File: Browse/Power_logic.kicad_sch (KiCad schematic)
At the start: 12 parts

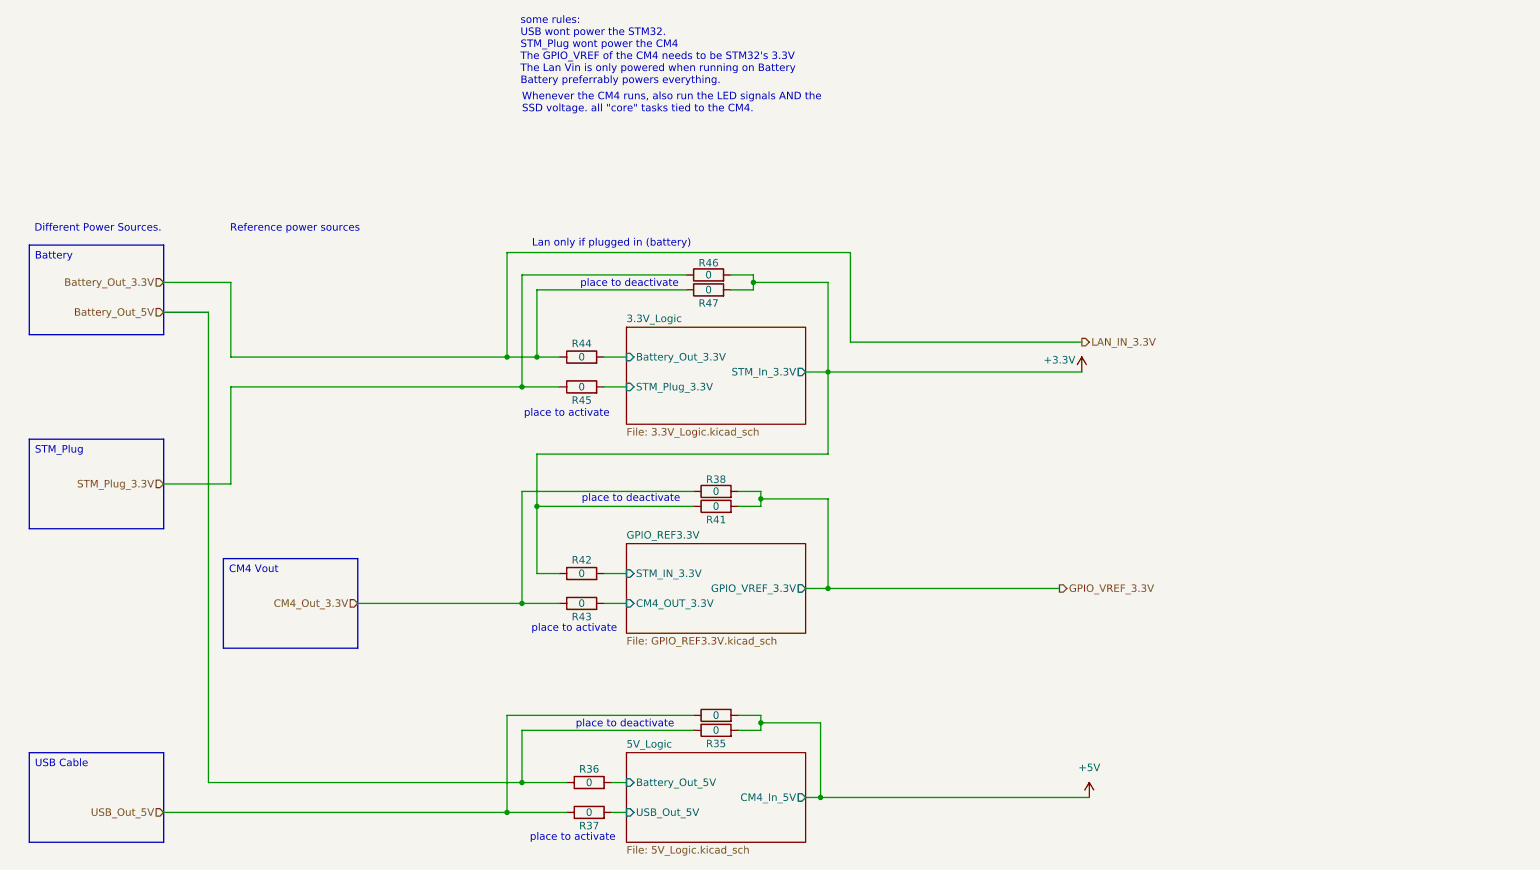
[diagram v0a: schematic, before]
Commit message: Deploying to gh-pages from @ Nautilus-UUV/nautilus-mainboard-PCB@5b07cf6af03655ef9ddad269b1edd5eb03bfa75f 🚀
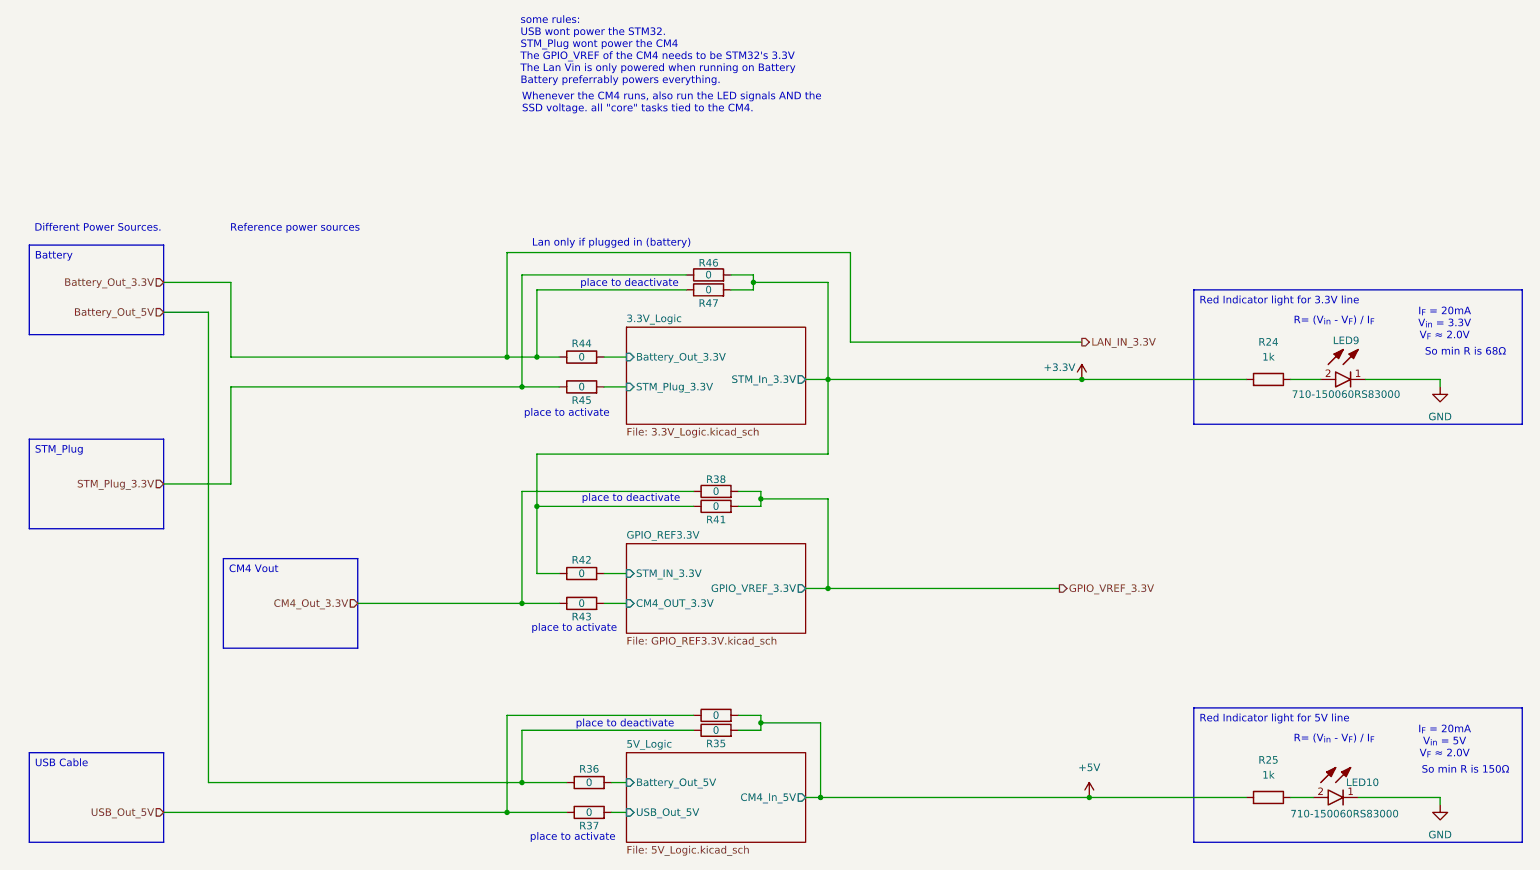
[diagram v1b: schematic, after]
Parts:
- added LED10, LED9: 710-150060RS83000, dz_dio:Wuerth_LED_150060RS83000, symbol #dzdb:s_dio/D-WURT-710-150060RS83000
- added R24, R25: 1k, Resistor_SMD:R_0603_1608Metric, symbol #dzdb:g_res/R-1k-0603
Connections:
- net +3.3V: now also R24.2
- net +5V: now also R25.2
- new net: LED10.2 (A), R25.1
- new net: LED9.2 (A), R24.1
- new net GND: LED10.1 (K), LED9.1 (K)
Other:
- note added: "I_{F} = 20mA V_{in} = 3.3V V_{F} ≈ 2.0V"
- note added: "I_{F} = 20mA V_{in} = 5V V_{F} ≈ 2.0V"
- note added: "R= (V_{in} - V_{F}) / I_{F}"
- note added: "So min R is 150Ω"
- note added: "So min R is 68Ω"
- title: (none) -> Nautilus_Mainboard
